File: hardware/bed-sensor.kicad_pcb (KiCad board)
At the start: 2 copper layers, 21.3 x 43.2 mm, 46 parts, among them J1 USB_B_Mini, J2 Conn_ARM_JTAG_SWD_10, J3 DM3AT-SF-PEJM5, J4 Conn_01x02, Q1 Q_PMOS_GSD, SW1 SW_Push, U1 MCP73831-2-OT, U2 TLV70218_SOT23-5, U3 AP2112K-3.3, U4 MDBT50Q-1M, U5 PCA9306, U6 ICM-20948, U7 BMP280, Y1 32.768

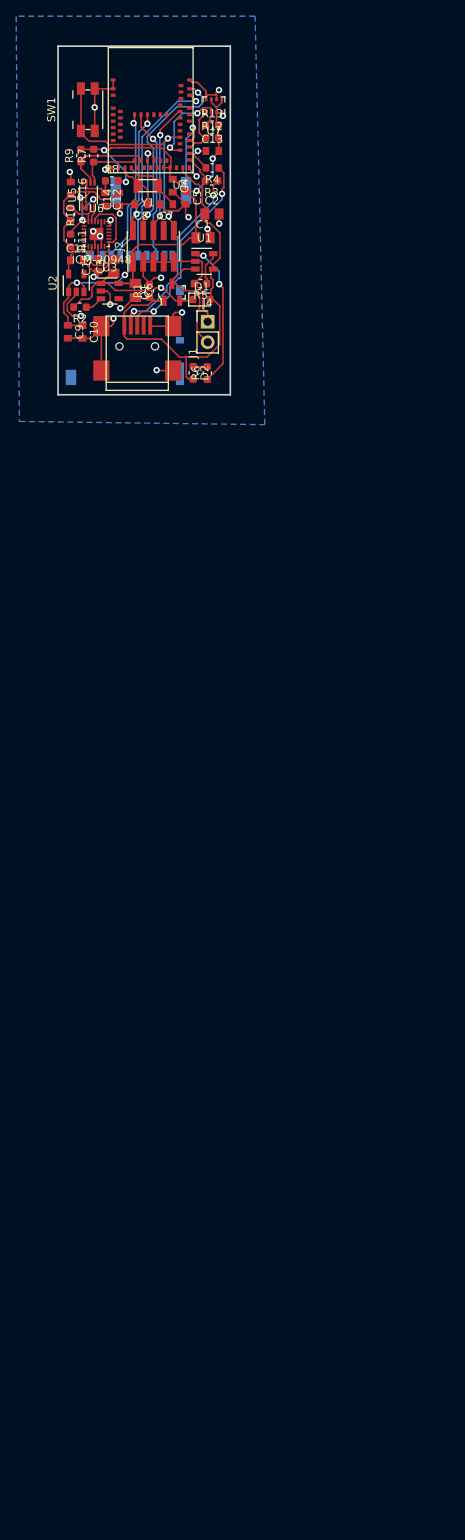
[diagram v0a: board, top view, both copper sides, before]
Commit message: tweaked board
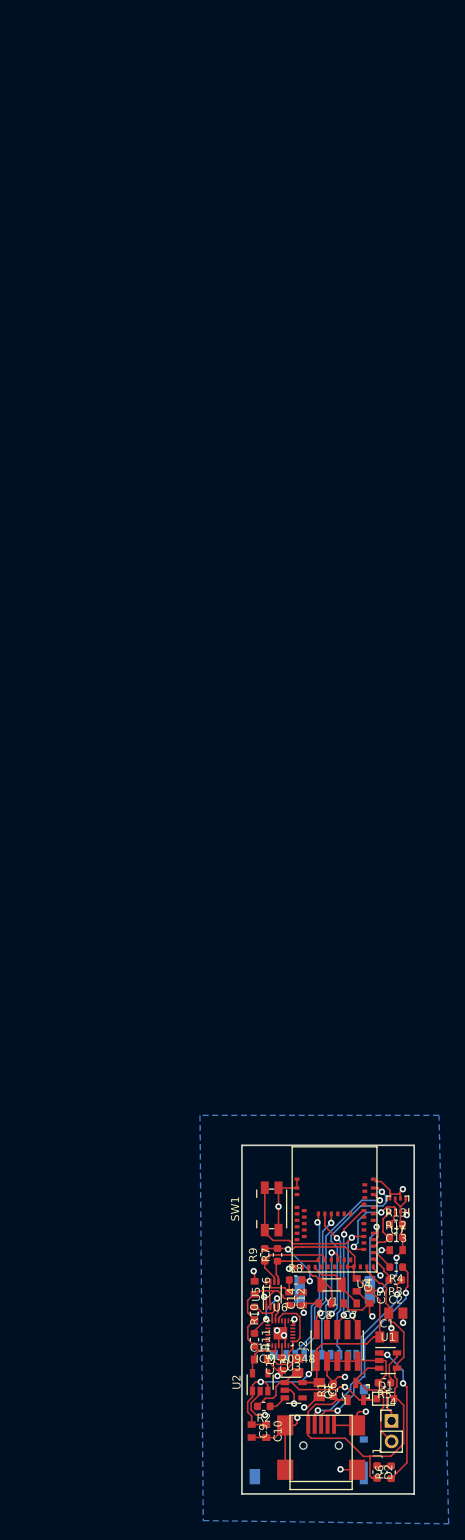
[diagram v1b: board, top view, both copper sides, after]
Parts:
- moved BZ1 138.0 mm to (148.1, 104.2)
- moved C1 138.0 mm to (154.5, 110.1)
- moved C10 138.0 mm to (139.6, 121.8)
- moved C11 138.0 mm to (138.9, 112.9)
- moved C12 138.0 mm to (142.4, 105.3)
- moved C14 138.0 mm to (144.1, 105.3)
- moved C15 138.0 mm to (141.5, 113.5)
- moved C16 138.0 mm to (138.1, 104.0)
- moved C2 138.0 mm to (155.6, 107.2)
- moved C3 138.0 mm to (143.5, 113.6)
- moved C4 138.0 mm to (150.8, 103.7)
- moved C5 138.0 mm to (152.4, 105.2)
- moved C6 138.0 mm to (146.1, 116.6)
- moved C7 138.0 mm to (150.0, 106.0)
- moved C8 138.0 mm to (146.9, 106.0)
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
